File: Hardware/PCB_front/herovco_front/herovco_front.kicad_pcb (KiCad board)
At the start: 2 copper layers, 94 x 125 mm, 80 parts, among them J101 3_pin_Molex_header, J102 Conn_01x06, J103 Conn_01x09, J104 Conn_01x07, J105 3_pin_Molex_connector, SW101 SW_SPDT_MSM, SW102 SW_Rotary12, U101 TL074, U102 AS3340A, U103 TL072, U104 TL431LP, U105 L79L05_TO92

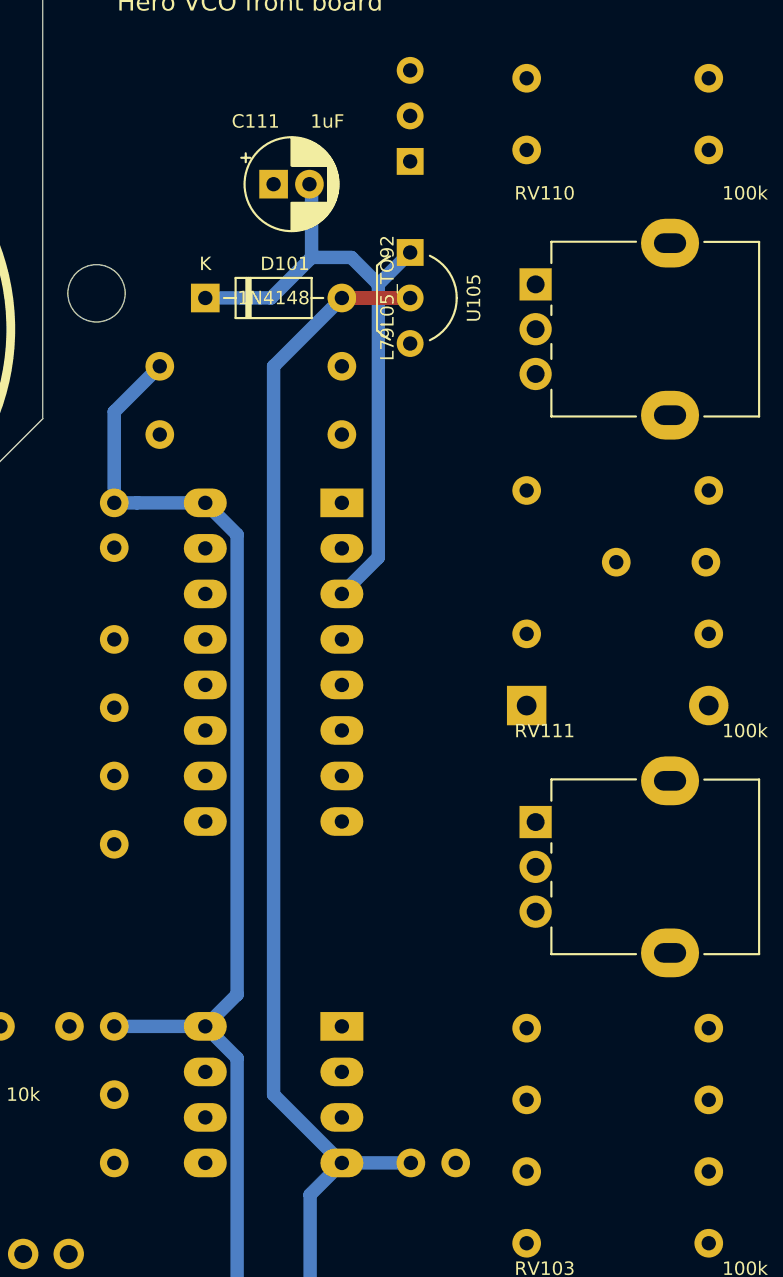
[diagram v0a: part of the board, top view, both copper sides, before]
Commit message: Change regulator output cap and rearrange
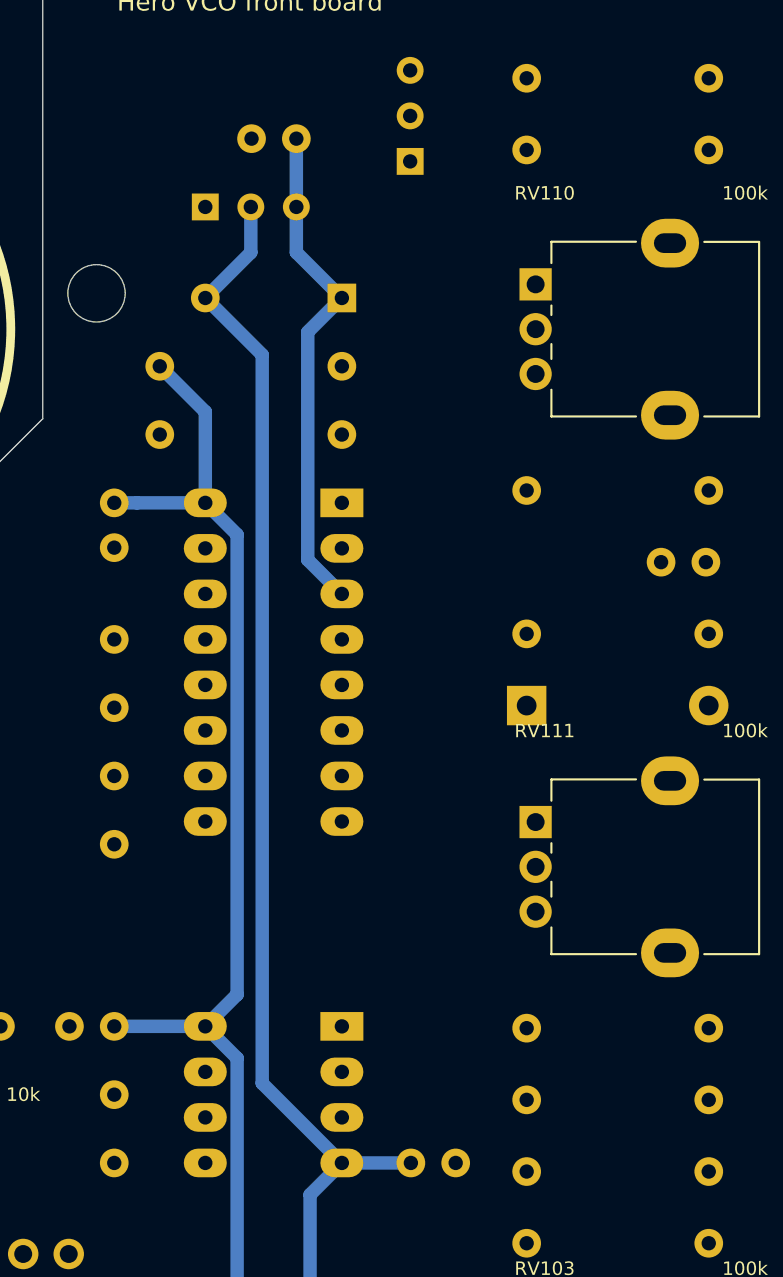
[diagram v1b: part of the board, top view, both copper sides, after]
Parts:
- C101: footprint ao_tht:C_Rect_L7.2mm_W2.5mm_P5.00mm_FKS2_FKP2_MKS2_MKP2 -> ao_tht:C_Disc_D3.0mm_W1.6mm_P2.50mm
- C111: value 1uF -> 10nF; footprint ao_tht:CP_Radial_D5.0mm_P2.00mm -> ao_tht:C_Disc_D3.0mm_W1.6mm_P2.50mm; moved to B.Cu
- D101, U105: moved to B.Cu
- moved U105 11.7 mm to (179.1, 43.2), turned to 0 degrees
- moved R120 10.2 mm to (197.0, 36.0), turned to 0 degrees
- moved R121 10.2 mm to (214.0, 39.0), turned to 0 degrees
- moved R122 10.2 mm to (197.0, 40.0), turned to 0 degrees
- moved D101 7.62 mm to (186.7, 48.3), turned to 180 degrees
- moved C111 2.82 mm to (181.7, 39.4)
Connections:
- R120 pad 1: Net-(R120-Pad1) -> +8V_REF
- R120 pad 2: +8V_REF -> Net-(R120-Pad2)
- R121 pad 1: GND -> Net-(R121-Pad1)
- R121 pad 2: Net-(R121-Pad2) -> GND
- R122 pad 1: +8V_REF -> +12V
- R122 pad 2: +12V -> +8V_REF
- RV107 pad 1: Net-(R121-Pad2) -> Net-(R121-Pad1)
- RV107 pad 3: Net-(R120-Pad1) -> Net-(R120-Pad2)
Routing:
- net -5V: track 35.8 -> 28.1 mm
- net -12V: track 102.9 -> 105.2 mm
